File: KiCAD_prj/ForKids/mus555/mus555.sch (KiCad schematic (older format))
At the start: 24 parts, among them J1 Screw_Terminal_01x02, SW1 SW_Push, SW2 SW_Push, SW3 SW_Push, SW4 SW_Push, SW5 SW_Push, SW6 SW_Push, SW7 SW_Push, SW8 SW_Push, U1 NE555

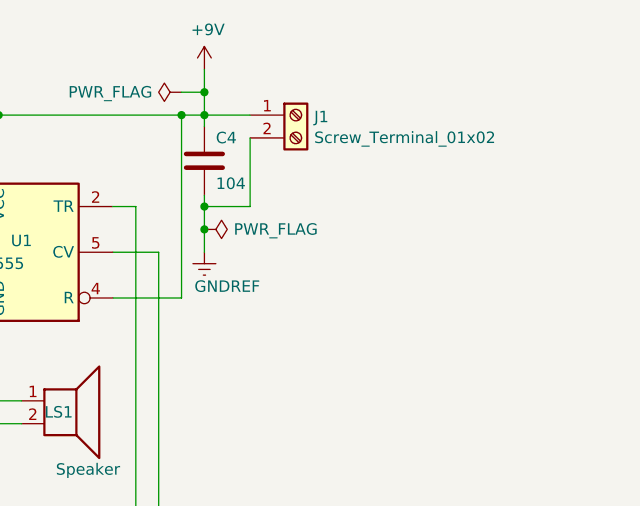
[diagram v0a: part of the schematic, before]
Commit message: Many changes
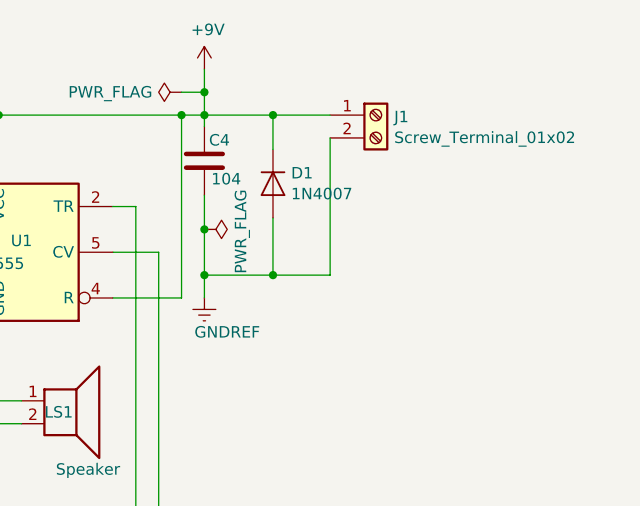
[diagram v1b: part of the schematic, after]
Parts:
- added D1: 1N4007, Diode_THT:D_DO-35_SOD27_P5.08mm_Vertical_AnodeUp, symbol Diode:1N4007
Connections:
- net +9V: now also D1.1 (K)
- net GNDREF: now also D1.2 (A)
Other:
- moved on the sheet: J1
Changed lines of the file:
@@
 L power:GNDREF #PWR0102
 U 1 1 5CC2759A
-P 8450 3500
-F 0 "#PWR0102" H 8450 3250 50  0001 C CNN
-F 1 "GNDREF" H 8550 3350 50  0000 C CNN
-F 2 "" H 8450 3500 50  0001 C CNN
-F 3 "" H 8450 3500 50  0001 C CNN
-	1    8450 3500
+P 8450 3700
+F 0 "#PWR0102" H 8450 3450 50  0001 C CNN
+F 1 "GNDREF" H 8550 3550 50  0000 C CNN
+F 2 "" H 8450 3700 50  0001 C CNN
+F 3 "" H 8450 3700 50  0001 C CNN
+	1    8450 3700
 	1    0    0    -1
 $EndComp
@@
 L Connector:Screw_Terminal_01x02 J1
 U 1 1 5CC2D610
-P 8850 2900
-F 0 "J1" H 8930 2892 50  0000 L CNN
-F 1 "Screw_Terminal_01x02" H 8930 2801 50  0000 L CNN
-F 2 "Connector_Phoenix_MC:PhoenixContact_MCV_1,5_2-G-3.5_1x02_P3.50mm_Vertical" H 8850 2900 50  0001 C CNN
-F 3 "~" H 8850 2900 50  0001 C CNN
-	1    8850 2900
+P 9200 2900
+F 0 "J1" H 9280 2892 50  0000 L CNN
+F 1 "Screw_Terminal_01x02" H 9280 2801 50  0000 L CNN
+F 2 "Connector_Phoenix_MC:PhoenixContact_MCV_1,5_2-G-3.5_1x02_P3.50mm_Vertical" H 9200 2900 50  0001 C CNN
+F 3 "~" H 9200 2900 50  0001 C CNN
+	1    9200 2900
 	1    0    0    -1
 $EndComp
@@
 Wire Wire Line
 	7700 4650 7700 4900
-Wire Wire Line
-	8450 3250 8450 3300
-Wire Wire Line
-	8650 3000 8650 3300
-Wire Wire Line
-	8650 3300 8450 3300
-Connection ~ 8450 3300
-Wire Wire Line
-	8450 3300 8450 3400
 $Comp
 L Device:C C1
@@
 P 8450 3400
 F 0 "#FLG0102" H 8450 3475 50  0001 C CNN
-F 1 "PWR_FLAG" V 8450 3528 50  0000 L CNN
+F 1 "PWR_FLAG" H 8275 3560 50  0000 L CNN
 F 2 "" H 8450 3400 50  0001 C CNN
 F 3 "~" H 8450 3400 50  0001 C CNN
@@
 	0    1    1    0
 $EndComp
-Connection ~ 8450 3400
-Wire Wire Line
-	8450 3500 8450 3400
 Wire Wire Line
 	7250 5300 7450 5300
@@
 $EndComp
 Wire Wire Line
-	8650 2900 8450 2900
-Wire Wire Line
 	6700 2900 6700 2950
 Wire Wire Line
@@
 Wire Wire Line
 	7550 2900 6700 2900
-Wire Wire Line
-	8450 2800 8450 2900
-Connection ~ 8450 2900
 Wire Wire Line
 	8450 2900 8350 2900
@@
 U 1 1 5CCD55A7
 P 8450 3100
-F 0 "C4" H 8500 3200 50  0000 L CNN
-F 1 "104" H 8500 3000 50  0000 L CNN
+F 0 "C4" H 8470 3190 50  0000 L CNN
+F 1 "104" H 8480 3020 50  0000 L CNN
 F 2 "Capacitor_THT:C_Disc_D4.7mm_W2.5mm_P5.00mm" H 8488 2950 50  0001 C CNN
 F 3 "~" H 8450 3100 50  0001 C CNN
@@
 	1    0    0    -1
 $EndComp
-Wire Wire Line
-	8450 2950 8450 2900
 Wire Wire Line
 	8050 3700 8350 3700
@@
 	0    -1   -1   0
 $EndComp
+Wire Wire Line
+	8450 3250 8450 3400
+Wire Wire Line
+	9000 3000 9000 3600
+Wire Wire Line
+	8450 2800 8450 2900
+Wire Wire Line
+	8450 3600 8450 3700
+Connection ~ 8450 3600
+Connection ~ 8450 3400
+Wire Wire Line
+	8450 3400 8450 3600
+Wire Wire Line
+	8450 3600 8750 3600
+Wire Wire Line
+	9000 2900 8750 2900
+Connection ~ 8450 2900
+Wire Wire Line
+	8450 2900 8450 2950
+$Comp
+L Diode:1N4007 D1
+U 1 1 5D3D4FB4
+P 8750 3200
+F 0 "D1" V 8704 3279 50  0000 L CNN
+F 1 "1N4007" V 8795 3279 50  0000 L CNN
+F 2 "Diode_THT:D_DO-35_SOD27_P5.08mm_Vertical_AnodeUp" H 8750 3025 50  0001 C CNN
+F 3 "http://www.vishay.com/docs/88503/1n4001.pdf" H 8750 3200 50  0001 C CNN
+	1    8750 3200
+	0    1    1    0
+$EndComp
+Wire Wire Line
+	8750 3050 8750 2900
+Connection ~ 8750 2900
+Wire Wire Line
+	8750 2900 8450 2900
+Wire Wire Line
+	8750 3350 8750 3600
+Connection ~ 8750 3600
+Wire Wire Line
+	8750 3600 9000 3600
 $EndSCHEMATC
